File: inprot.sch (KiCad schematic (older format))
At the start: 3 parts

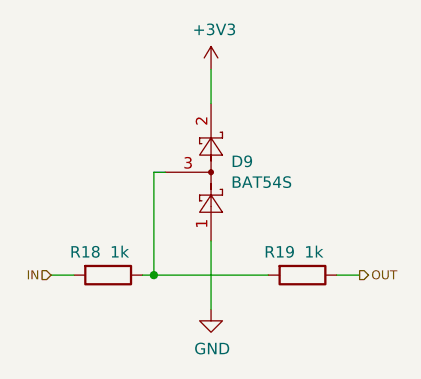
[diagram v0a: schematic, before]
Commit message: Closes #14
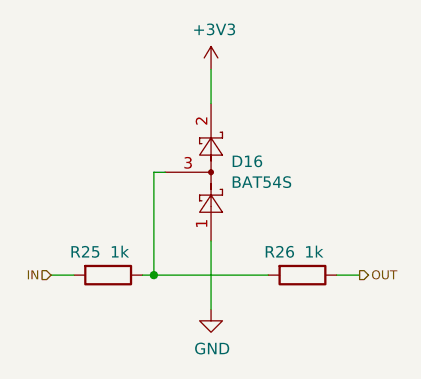
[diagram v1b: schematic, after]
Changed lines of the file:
@@
 AR Path="/612F6239/60E60B36" Ref="D15"  Part="1"
 AR Path="/6132323D/60E60B36" Ref="D16"  Part="1"
-F 0 "D9" V 6046 3238 50  0000 L CNN
+F 0 "D16" V 6046 3238 50  0000 L CNN
 F 1 "BAT54S" V 5955 3238 50  0000 L CNN
 F 2 "Package_TO_SOT_SMD:SOT-23" H 6075 3275 50  0001 L CNN
@@
 AR Path="/612F6239/60E62337" Ref="R23"  Part="1"
 AR Path="/6132323D/60E62337" Ref="R25"  Part="1"
-F 0 "R18" V 5450 3500 50  0000 C CNN
+F 0 "R25" V 5450 3500 50  0000 C CNN
 F 1 "1k" V 5450 3650 50  0000 C CNN
 F 2 "Resistor_SMD:R_1206_3216Metric" V 5480 3600 50  0001 C CNN
@@
 AR Path="/612F6239/60E62A46" Ref="R24"  Part="1"
 AR Path="/6132323D/60E62A46" Ref="R26"  Part="1"
-F 0 "R19" V 6300 3500 50  0000 C CNN
+F 0 "R26" V 6300 3500 50  0000 C CNN
 F 1 "1k" V 6300 3650 50  0000 C CNN
 F 2 "Resistor_SMD:R_1206_3216Metric" V 6330 3600 50  0001 C CNN
@@
 AR Path="/612F6239/60E632B2" Ref="#PWR0136"  Part="1"
 AR Path="/6132323D/60E632B2" Ref="#PWR0142"  Part="1"
-F 0 "#PWR055" H 6000 3500 50  0001 C CNN
+F 0 "#PWR0142" H 6000 3500 50  0001 C CNN
 F 1 "GND" H 6005 3577 50  0000 C CNN
 F 2 "" H 6000 3750 50  0001 C CNN
@@
 AR Path="/612F6239/60E63A61" Ref="#PWR0137"  Part="1"
 AR Path="/6132323D/60E63A61" Ref="#PWR0143"  Part="1"
-F 0 "#PWR054" H 6000 2550 50  0001 C CNN
+F 0 "#PWR0143" H 6000 2550 50  0001 C CNN
 F 1 "+3V3" H 6015 2873 50  0000 C CNN
 F 2 "" H 6000 2700 50  0001 C CNN

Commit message: Closes #13
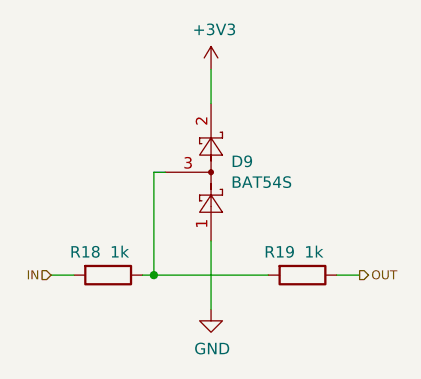
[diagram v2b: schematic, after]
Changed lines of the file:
@@
 AR Path="/612F6239/60E60B36" Ref="D15"  Part="1"
 AR Path="/6132323D/60E60B36" Ref="D16"  Part="1"
-F 0 "D16" V 6046 3238 50  0000 L CNN
+F 0 "D9" V 6046 3238 50  0000 L CNN
 F 1 "BAT54S" V 5955 3238 50  0000 L CNN
 F 2 "Package_TO_SOT_SMD:SOT-23" H 6075 3275 50  0001 L CNN
@@
 AR Path="/612F6239/60E62337" Ref="R23"  Part="1"
 AR Path="/6132323D/60E62337" Ref="R25"  Part="1"
-F 0 "R25" V 5450 3500 50  0000 C CNN
+F 0 "R18" V 5450 3500 50  0000 C CNN
 F 1 "1k" V 5450 3650 50  0000 C CNN
 F 2 "Resistor_SMD:R_1206_3216Metric" V 5480 3600 50  0001 C CNN
@@
 AR Path="/612F6239/60E62A46" Ref="R24"  Part="1"
 AR Path="/6132323D/60E62A46" Ref="R26"  Part="1"
-F 0 "R26" V 6300 3500 50  0000 C CNN
+F 0 "R19" V 6300 3500 50  0000 C CNN
 F 1 "1k" V 6300 3650 50  0000 C CNN
 F 2 "Resistor_SMD:R_1206_3216Metric" V 6330 3600 50  0001 C CNN
@@
 AR Path="/612F6239/60E632B2" Ref="#PWR0136"  Part="1"
 AR Path="/6132323D/60E632B2" Ref="#PWR0142"  Part="1"
-F 0 "#PWR0142" H 6000 3500 50  0001 C CNN
+F 0 "#PWR055" H 6000 3500 50  0001 C CNN
 F 1 "GND" H 6005 3577 50  0000 C CNN
 F 2 "" H 6000 3750 50  0001 C CNN
@@
 AR Path="/612F6239/60E63A61" Ref="#PWR0137"  Part="1"
 AR Path="/6132323D/60E63A61" Ref="#PWR0143"  Part="1"
-F 0 "#PWR0143" H 6000 2550 50  0001 C CNN
+F 0 "#PWR054" H 6000 2550 50  0001 C CNN
 F 1 "+3V3" H 6015 2873 50  0000 C CNN
 F 2 "" H 6000 2700 50  0001 C CNN
